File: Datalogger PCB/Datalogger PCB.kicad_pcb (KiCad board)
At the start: 4 copper layers, 42.2 x 102 mm, 21 parts, among them J1 Conn_01x02_Pin, U2 W25Q128JVS

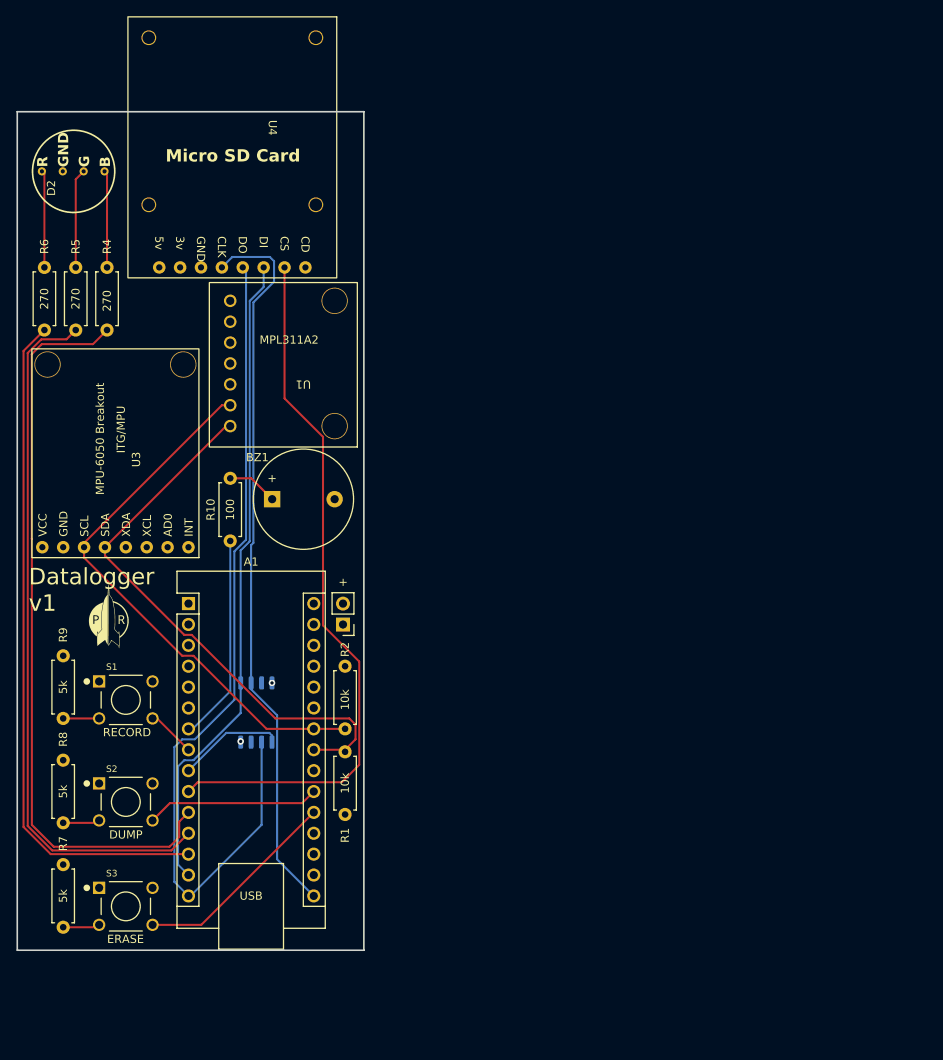
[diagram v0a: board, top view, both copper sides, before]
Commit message: V2 pcb (#19)
Completed PCB design
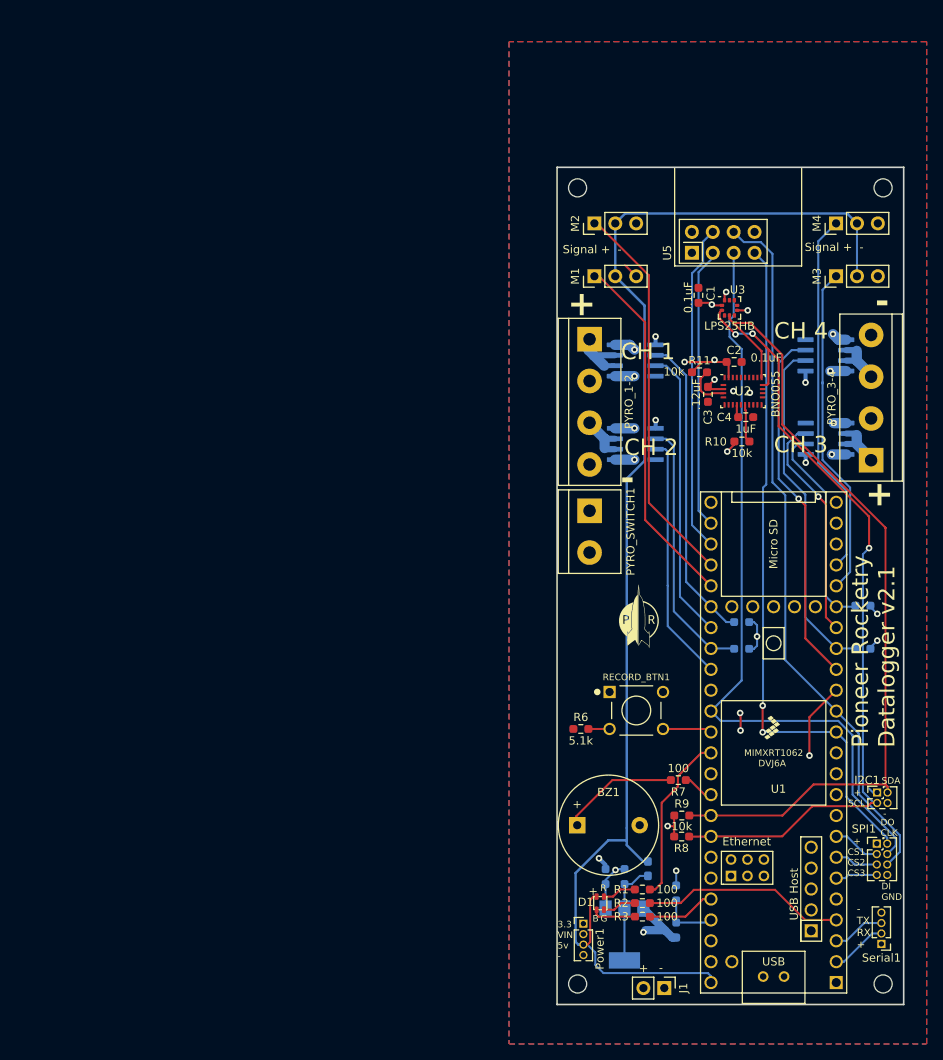
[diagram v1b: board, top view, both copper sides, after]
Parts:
- removed A1: Arduino_Nano_v3.x, Module:Arduino_Nano
- removed S1, S2, S3: FSM8JH, Push Button:SW_FSM8JH
- added C1: 0.1uF, Resistor_SMD:R_0603_1608Metric_Pad0.98x0.95mm_HandSolder, F.Cu at (154.7, 57.8)
- added C2: 0.1uF, Resistor_SMD:R_0603_1608Metric_Pad0.98x0.95mm_HandSolder, F.Cu at (159.1, 65.9)
- added C3: .12uF, Resistor_SMD:R_0603_1608Metric_Pad0.98x0.95mm_HandSolder, F.Cu at (155.9, 69.8)
- added C4: 1uF, Resistor_SMD:R_0603_1608Metric_Pad0.98x0.95mm_HandSolder, F.Cu at (160.5, 72.6)
- added C5: 10uF, Resistor_SMD:R_0603_1608Metric_Pad0.98x0.95mm_HandSolder, B.Cu at (143.4, 128.5)
- added C6: 22uF, Resistor_SMD:R_0603_1608Metric_Pad0.98x0.95mm_HandSolder, B.Cu at (145.8, 128.5)
- added D1: LED_GBAR, Led:LED_GBAR, F.Cu at (143.2, 132.5)
- added H1: MountingHole, MountingHole:MountingHole_2.2mm_M2, F.Cu at (140.0, 44.7)
- added H2: MountingHole, MountingHole:MountingHole_2.2mm_M2, F.Cu at (177.2, 44.7)
- added H3: MountingHole, MountingHole:MountingHole_2.2mm_M2, F.Cu at (177.2, 141.5)
- added H4: MountingHole, MountingHole:MountingHole_2.2mm_M2, F.Cu at (140.0, 141.5)
- added I2C1: Conn_02x02_Counter_Clockwise, Connector_PinHeader_1.27mm:PinHeader_2x02_P1.27mm_Vertical, F.Cu at (176.5, 118.2)
- added M1: Motor_Servo, Connector_PinHeader_2.54mm:PinHeader_1x03_P2.54mm_Vertical, F.Cu at (142.1, 55.4)
- added M2: Motor_Servo, Connector_PinHeader_2.54mm:PinHeader_1x03_P2.54mm_Vertical, F.Cu at (142.1, 49.0)
- added M3: Motor_Servo, Connector_PinHeader_2.54mm:PinHeader_1x03_P2.54mm_Vertical, F.Cu at (171.5, 55.4)
- added M4: Motor_Servo, Connector_PinHeader_2.54mm:PinHeader_1x03_P2.54mm_Vertical, F.Cu at (171.5, 49.0)
- added PYRO_1-2: Screw_Terminal_01x04, TerminalBlock:TerminalBlock_bornier-4_P5.08mm, F.Cu at (141.5, 63.1)
- added PYRO_3-4: Screw_Terminal_01x04, TerminalBlock:TerminalBlock_bornier-4_P5.08mm, F.Cu at (175.8, 77.8)
- added PYRO_SWITCH1: Screw_Terminal_01x02, TerminalBlock:TerminalBlock_bornier-2_P5.08mm, F.Cu at (141.5, 84.0)
- added Power1: Conn_01x04_Pin, Connector_PinHeader_1.27mm:PinHeader_1x04_P1.27mm_Vertical, F.Cu at (140.8, 134.2)
- added R11: 10k, Resistor_SMD:R_0603_1608Metric_Pad0.98x0.95mm_HandSolder, F.Cu at (154.9, 67.1)
- added R12: 10k, Resistor_SMD:R_0603_1608Metric_Pad0.98x0.95mm_HandSolder, B.Cu at (152.0, 135.0)
- added R13: 2k, Resistor_SMD:R_0603_1608Metric_Pad0.98x0.95mm_HandSolder, B.Cu at (152.0, 130.4)
- added R14: 10k, Resistor_SMD:R_0603_1608Metric_Pad0.98x0.95mm_HandSolder, B.Cu at (174.8, 95.5)
- added R15: 10k, Resistor_SMD:R_0603_1608Metric_Pad0.98x0.95mm_HandSolder, B.Cu at (174.8, 100.8)
- added R3: 100, Resistor_SMD:R_0603_1608Metric_Pad0.98x0.95mm_HandSolder, F.Cu at (147.9, 133.3)
- added RECORD_BTN1: FSM8JH, Push Button:SW_FSM8JH, F.Cu at (147.2, 108.3)
- added SPI1: Conn_02x04_Counter_Clockwise, Connector_PinHeader_1.27mm:PinHeader_2x04_P1.27mm_Vertical, F.Cu at (176.4, 124.5)
- added Serial1: Conn_01x04_Pin, Connector_PinHeader_1.27mm:PinHeader_1x04_P1.27mm_Vertical, F.Cu at (177.0, 136.7)
- added U5: NRF24L01_Breakout, RF_Module:nRF24L01_Breakout, F.Cu at (153.9, 52.6)
- added U6: VN5E160STR-E, SOIC127P600X175-8N:SOIC127P600X175-8N, B.Cu at (147.1, 65.7)
- added U7: VN5E160STR-E, SOIC127P600X175-8N:SOIC127P600X175-8N, B.Cu at (147.1, 75.8)
- added U8: VN5E160STR-E, SOIC127P600X175-8N:SOIC127P600X175-8N, B.Cu at (170.3, 75.2)
- added U9: VN5E160STR-E, SOIC127P600X175-8N:SOIC127P600X175-8N, B.Cu at (170.2, 65.1)
- D2: value LED_RKGB -> D; footprint Breakout Boards:RGB_LED -> Diode_SMD:D_0603_1608Metric_Pad1.05x0.95mm_HandSolder; moved to B.Cu
- R1, R2: value 10k -> 100; footprint Resistor_THT:R_Axial_DIN0207_L6.3mm_D2.5mm_P7.62mm_Horizontal -> Resistor_SMD:R_0603_1608Metric_Pad0.98x0.95mm_HandSolder
- R10: value 100 -> 10k; footprint Resistor_THT:R_Axial_DIN0207_L6.3mm_D2.5mm_P7.62mm_Horizontal -> Resistor_SMD:R_0603_1608Metric_Pad0.98x0.95mm_HandSolder
- R4, R5: value 270 -> 10k; footprint Resistor_THT:R_Axial_DIN0207_L6.3mm_D2.5mm_P7.62mm_Horizontal -> Resistor_SMD:R_0603_1608Metric_Pad0.98x0.95mm_HandSolder; moved to B.Cu
- R6: value 270 -> 5.1k; footprint Resistor_THT:R_Axial_DIN0207_L6.3mm_D2.5mm_P7.62mm_Horizontal -> Resistor_SMD:R_0603_1608Metric_Pad0.98x0.95mm_HandSolder
- R7: value 5k -> 100; footprint Resistor_THT:R_Axial_DIN0207_L6.3mm_D2.5mm_P7.62mm_Horizontal -> Resistor_SMD:R_0603_1608Metric_Pad0.98x0.95mm_HandSolder
- R8, R9: value 5k -> 10k; footprint Resistor_THT:R_Axial_DIN0207_L6.3mm_D2.5mm_P7.62mm_Horizontal -> Resistor_SMD:R_0603_1608Metric_Pad0.98x0.95mm_HandSolder
- U1: value ~ -> Teensy4.1; footprint Breakout Boards:MPL3115A2 -> Teensy4.1:Teensy41
- U2: value W25Q128JVS -> BNO055; footprint Package_SO:SOIC-8_5.23x5.23mm_P1.27mm -> Package_LGA:LGA-28_5.2x3.8mm_P0.5mm; moved to F.Cu
- U3: value ~ -> LPS25HB; footprint Datalogging Breakout:MPU-6050 Breakout -> Package_LGA:ST_HLGA-10_2.5x2.5mm_P0.6mm_LayoutBorder3x2y
- U4: value ~ -> AMS1117-5.0; footprint Breakout Boards:Adafruit Micro-SD Breakout Board+ -> Package_TO_SOT_SMD:SOT-223-3_TabPin2; moved to B.Cu
- moved D2 112.4 mm to (148.6, 127.5), turned to -90 degrees
- moved U3 93.2 mm to (158.5, 59.3), turned to 0 degrees
- moved U4 90.0 mm to (145.7, 135.5)
- moved R5 88.5 mm to (160.0, 97.5), turned to 180 degrees
- moved R4 86.4 mm to (160.0, 100.8), turned to 180 degrees
- moved R6 81.3 mm to (140.4, 110.5), turned to 0 degrees
- moved R9 77.7 mm to (152.7, 121.0), turned to 0 degrees
- moved U1 77.5 mm to (163.9, 112.1), turned to 90 degrees
- moved R8 75.8 mm to (152.7, 123.6), turned to 0 degrees
- moved R7 75.5 mm to (152.3, 116.7), turned to 180 degrees
- moved U2 70.9 mm to (160.2, 69.4), turned to 0 degrees
- moved G*** 64.5 mm to (147.4, 96.6)
- moved R10 63.4 mm to (160.0, 75.5), turned to 0 degrees
- moved J1 59.0 mm to (150.6, 142.0), turned to -90 degrees
- moved BZ1 54.3 mm to (140.0, 122.2)
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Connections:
- D2 pad 1: Net-(D2-RA) -> +5V
- D2 pad 2: GND -> Net-(D2-A)
- J1 pad 2: Net-(A1-VIN) -> /VIN
- R1 pad 1: +5V -> /RGB-R
- R1 pad 2: SDA -> Net-(D1-RK)
- R10 pad 1: Net-(A1-D4) -> +3.3V
- R10 pad 2: Net-(BZ1--) -> Net-(U2-~{RESET})
- R2 pad 1: +5V -> /RGB-G
- R2 pad 2: SCL -> Net-(D1-GK)
- R4 pad 1: RGB-B -> GND
- R4 pad 2: Net-(D2-BA) -> /PYRO_2
- R5 pad 1: RGB-G -> GND
- R5 pad 2: Net-(D2-GA) -> /PYRO_1
- R6 pad 1: RGB-R -> GND
- R6 pad 2: Net-(D2-RA) -> Net-(R6-Pad2)
- R7 pad 1: GND -> Net-(U1-17_A3_TX4_SDA1)
- R7 pad 2: Net-(R7-Pad2) -> Net-(BZ1--)
- R8 pad 1: GND -> +3.3V
- R8 pad 2: Net-(R8-Pad2) -> /SCL
- R9 pad 1: GND -> +3.3V
- R9 pad 2: Net-(R9-Pad2) -> /SDA
- U1 pad 1: SDA -> GND
- U1 pad 2: SCL -> /RX
- U1 pad 3: unconnected-(U1-INT1-Pad3) -> /TX
- U1 pad 4: unconnected-(U1-INT2-Pad4) -> /RGB-G
- U1 pad 6: GND -> /EXTERNAL_CS3
- U1 pad 7: +5V -> /EXTERNAL_CS2
- U1 pad 8: (no net) -> /EXTERNAL_CS1
- U1 pad 9: (no net) -> unconnected-(U1-7_RX2_OUT1A-Pad9)
- U2 pad 1: FLASH_CS -> unconnected-(U2-PIN1-Pad1)
- U2 pad 2: DO -> GND
- U2 pad 3: unconnected-(U2-IO2-Pad3) -> +3.3V
- U2 pad 4: GND -> Net-(U2-~{BOOT_LOAD_PIN})
- U2 pad 5: DI -> GND
- U2 pad 6: CLK -> GND
- U2 pad 8: +3V3 -> unconnected-(U2-PIN8-Pad8)
- U3 pad 1: +5V -> +3.3V
- U3 pad 10: (no net) -> +3.3V
- U3 pad 2: GND -> /SCL
- U3 pad 3: SCL -> unconnected-(U3-RES-Pad3)
- U3 pad 4: SDA -> /SDA
- U3 pad 6: unconnected-(U3-XDL-Pad6) -> +3.3V
- U3 pad 8: unconnected-(U3-INT-Pad8) -> GND
- U3 pad 9: (no net) -> GND
- U4 pad 1: unconnected-(U4-CD-Pad1) -> GND
- U4 pad 2: SD_CS -> Net-(D2-A)
- U4 pad 3: DI -> /VIN
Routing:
- net +5V: track 0.00 -> 161.4 mm
- net DO: track 104.4 -> 0.00 mm
- net /SDA: track 0.00 -> 100.7 mm
- net /SCL: track 0.00 -> 100.2 mm, vias 0 -> 3
- net +3V3: track 100.1 -> 0.00 mm, vias 1 -> 0
- net /CLK: track 0.00 -> 93.6 mm
- net RGB-B: track 90.6 -> 0.00 mm
- net CLK: track 88.6 -> 0.00 mm
- net /PYRO_POWER: track 0.00 -> 87.4 mm, vias 0 -> 8
- net /DI: track 0.00 -> 87.2 mm
- net SD_CS: track 86.4 -> 0.00 mm
- net RGB-G: track 86.2 -> 0.00 mm
- net /DO: track 0.00 -> 84.2 mm, vias 0 -> 2
- net RGB-R: track 82.9 -> 0.00 mm
- net DI: track 79.4 -> 0.00 mm
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- added copper zone on B.Cu, net +3.3V
- added copper zone on In2.Cu, net +3.3V
- added copper zone on F.Cu, net GND
- added copper zone on In1.Cu, net GND
- removed copper zone on In1.Cu, net +5V
- removed copper zone on In2.Cu, net GND
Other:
- board size 42.2 x 102 mm -> 42.2 x 101.8 mm
- board text added: "+ CS1 CS2 CS3"
- board text added: "+ SCL"
- board text added: "-"
- board text added: "- TX RX +"
- board text added: "3.3 VIN 5v -"
- board text added: "CH 1"
- board text added: "CH 2"
- board text added: "CH 3"
- board text added: "CH 4"
- board text added: "DI GND"
- board text added: "DO CLK"
- board text added: "Pioneer Rocketry Datalogger v2.1"
- board text added: "SDA"
- board text added: "Signal + -"
- board text removed: "DUMP"
- board text removed: "Datalogger v1"
- board text removed: "Developed By Pioneer Rocketry"
- board text removed: "ERASE"
- board text removed: "MPL311A2"
- board text removed: "Micro SD Card"
- board text removed: "RECORD"
